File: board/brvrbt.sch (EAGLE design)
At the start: 9 parts, among them IC1 7805

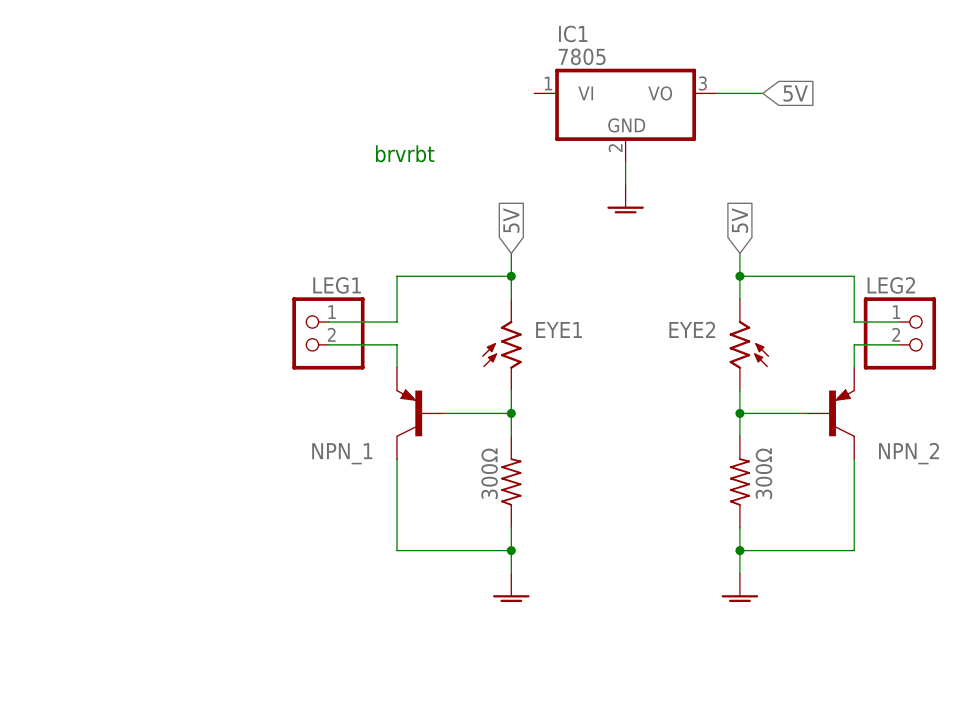
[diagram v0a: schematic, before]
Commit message: silk work
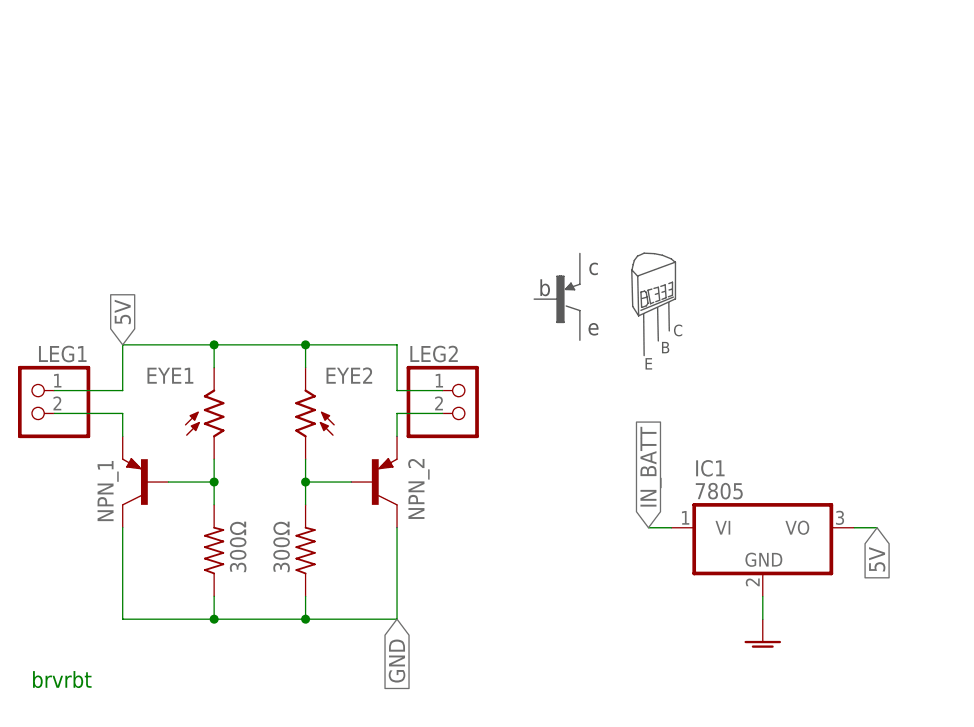
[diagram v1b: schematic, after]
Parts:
- NPN_2: value (none) -> E B C
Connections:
- new net IN_BATT: IC1.VI
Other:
- note added: "B"
- note added: "C"
- note added: "E"
- note added: "b"
- note added: "c"
- note added: "e"
- moved on the sheet: EYE1, EYE2, IC1, LEG1, LEG2, NPN_1, NPN_2
